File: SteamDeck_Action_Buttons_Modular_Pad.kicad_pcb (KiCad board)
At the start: 2 copper layers, 50.2 x 32.1 mm, 15 parts

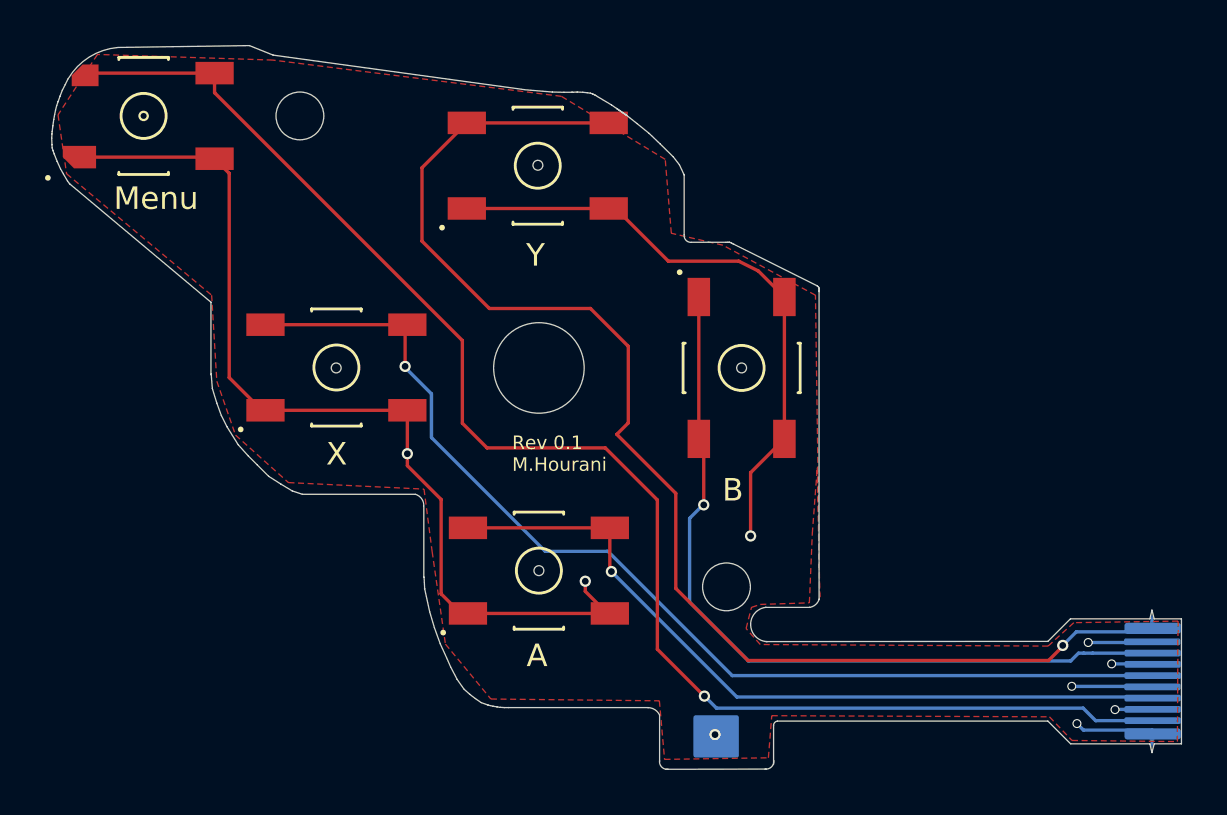
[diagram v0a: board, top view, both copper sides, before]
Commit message: rev 0.2
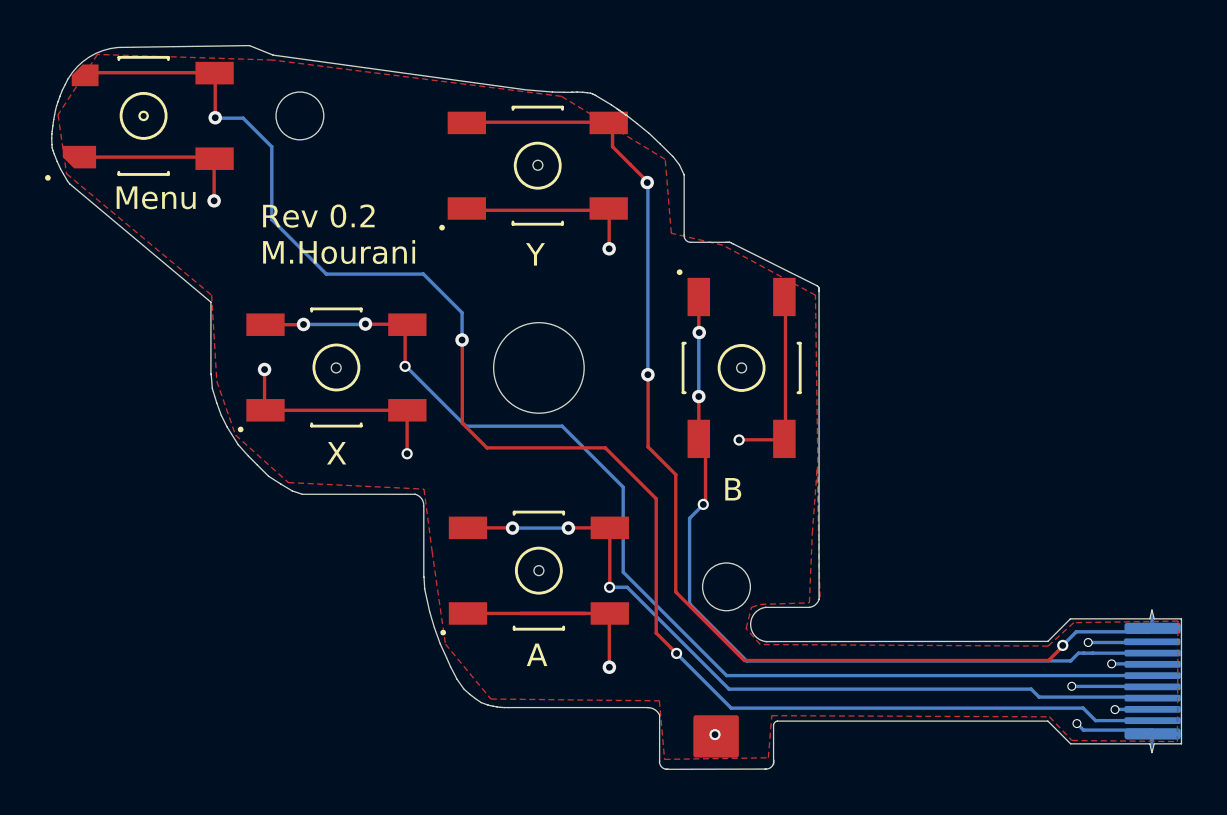
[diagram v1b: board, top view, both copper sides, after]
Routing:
- net GND: track 86.4 -> 59.4 mm, vias 9 -> 12
- net Y-Button: track 58.6 -> 51.3 mm, vias 1 -> 3
- net Menu-Button: track 65.7 -> 68.6 mm, vias 1 -> 3
- net X-Button: track 47.9 -> 49.3 mm, vias 1 -> 3
- net A-Button: track 34.4 -> 34.9 mm, vias 1 -> 3
- net B-Button: track 35.5 -> 35.7 mm, vias 1 -> 3
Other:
- board text added: "Rev 0.2 M.Hourani"
- board text removed: "Rev 0.1 M.Hourani"
